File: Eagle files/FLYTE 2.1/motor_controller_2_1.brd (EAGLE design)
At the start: 80 x 53.6 mm, 38 parts, among them J1 XT60-M, U1 MIC29302WU-TRTO-263-5_MCH-M, U2 MIC29302WU-TRTO-263-5_MCH-M

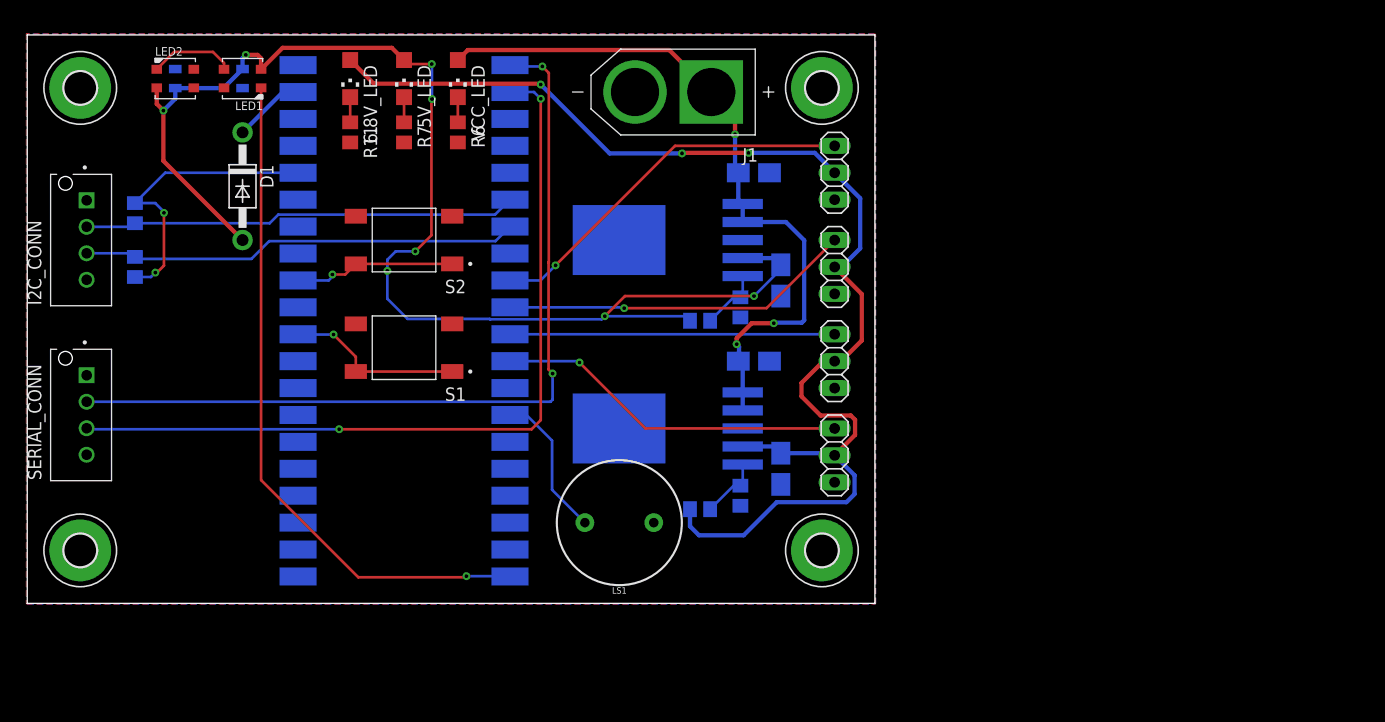
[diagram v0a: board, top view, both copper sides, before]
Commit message: motor controller v2.1
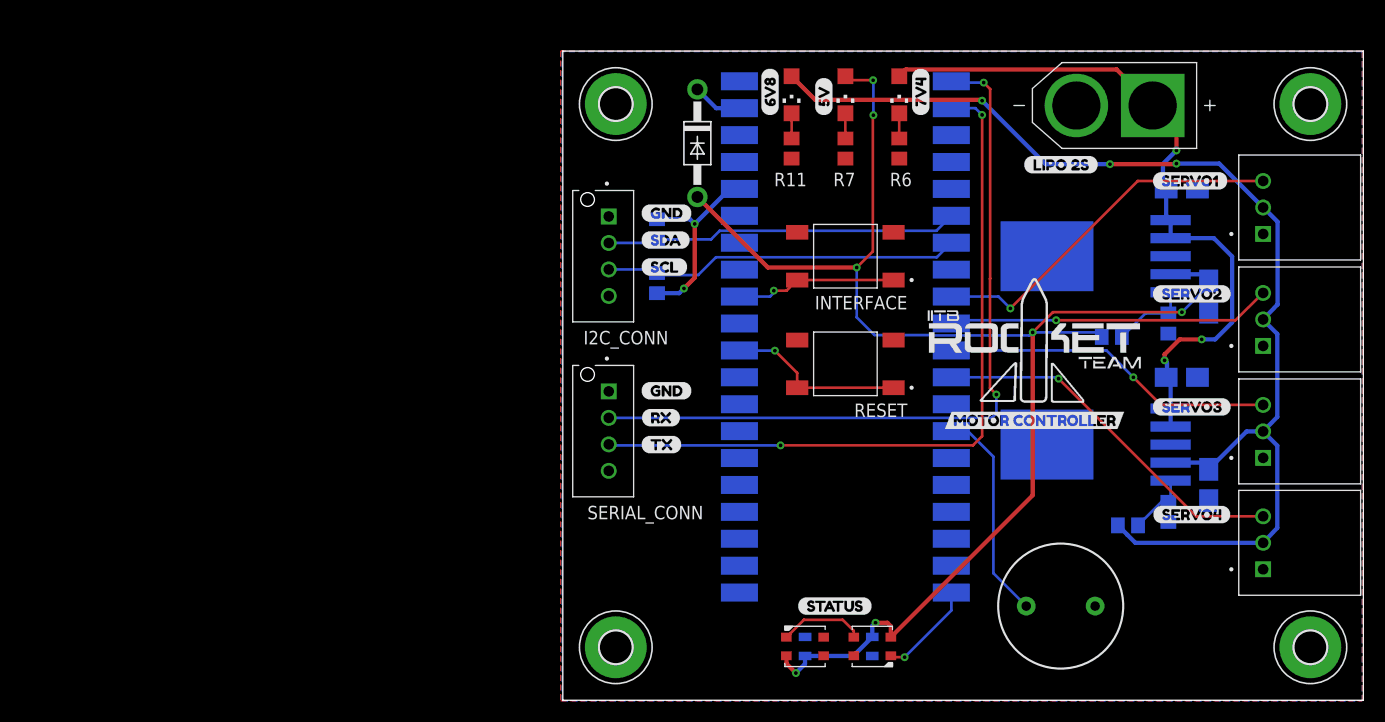
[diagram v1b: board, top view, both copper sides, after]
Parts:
- removed S1, S2: TS04-66-95-BK-100-SMT, TS04-66-95-BK-100-SMT:SW_TS04-66-95-BK-100-SMT
- removed SERVO1, SERVO2, SERVO3, SERVO4: (no value), pinhead:1X03
- added INTERFACE, RESET: TS04-66-95-BK-100-SMT, TS04-66-95-BK-100-SMT:SW_TS04-66-95-BK-100-SMT
- added J2, J3, J4, J5: S3B-XH-A(LF)(SN), S3B-XH-A_LF__SN_:JST_S3B-XH-A(LF)(SN)
- added U$1: (no value), servo1_label:SERVO10
- added U$10: (no value), tx_label:TX0
- added U$11: (no value), lipo_2s_label:LIPO_2S0
- added U$12: (no value), 5v_label:5V0
- added U$13: (no value), 7v4_label:7V40
- added U$14: (no value), 6v8_label:6V80
- added U$15: (no value), status_label:STATUS0
- added U$16: (no value), motor_controller_label:MOTOR_CONTROLLER0
- added U$2: (no value), servo2_label:SERVO20
- added U$3: (no value), servo3_label:SERVO30
- added U$4: (no value), servo4_label:SERVO40
- added U$5: (no value), sda_label:SDA0
- added U$6: (no value), scl_label:SCL0
- added U$7, U$8: (no value), gnd_label:GND0
- added U$9: (no value), rx_label:RX0
- moved C4 80.0 mm to (73.4, 2.29)
- moved LED2 80.0 mm to (73.4, 2.29)
- moved C3 80.0 mm to (79.8, 2.29)
- moved LED1 80.0 mm to (79.8, 2.29)
- moved H3 51.4 mm to (55.5, 2.21)
- moved H2 50.6 mm to (55.5, 53.5)
- moved I2C_CONN 49.3 mm to (54.4, 39.1)
- moved SERIAL_CONN 49.3 mm to (54.4, 22.6)
- moved R3 49.3 mm to (59.4, 36.6)
- moved R4 49.3 mm to (59.4, 41.7)
- moved H4 47.0 mm to (121.1, 2.21)
- moved H1 46.1 mm to (121.1, 53.5)
- moved D1 43.1 mm to (63.2, 49.8)
- moved LS1 42.4 mm to (97.5, 6.10)
- moved PICO 41.7 mm to (78.5, 30.2)
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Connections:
- net 6.8V: now also J2.2, J3.2, J4.2, J5.2; no longer SERVO1.2, SERVO2.2, SERVO3.2, SERVO4.2
- net GND: now also INTERFACE.2, INTERFACE.4, J2.1, J3.1, J4.1, J5.1, RESET.2, RESET.4; no longer S1.2, S1.4, S2.2, S2.4, SERVO1.1, SERVO2.1, SERVO3.1, SERVO4.1
- net N$2: now also RESET.1, RESET.3; no longer S1.1, S1.3
- net N$3: now also INTERFACE.1, INTERFACE.3; no longer S2.1, S2.3
- net SERVO1: now also J2.3; no longer SERVO1.3
- net SERVO2: now also J3.3; no longer SERVO2.3
- net SERVO3: now also J4.3; no longer SERVO3.3
- net SERVO4: now also J5.3; no longer SERVO4.3
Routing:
- net LED: track 65.7 -> 9.28 mm
- net 5V: track 126.4 -> 139.9 mm, vias 8 -> 7
- net 6.8V: track 120.8 -> 109.6 mm
- net 3V3: track 28.0 -> 18.6 mm
- net SDA0: track 41.0 -> 33.4 mm
- net SCL0: track 41.4 -> 33.8 mm
- net SER_RX: track 76.7 -> 69.1 mm
- net SER_TX: track 79.0 -> 71.6 mm
- net BUZZER: track 14.0 -> 20.4 mm
- net SERVO2: track 33.3 -> 30.6 mm
- net N$1: track 6.82 -> 4.71 mm
- net SERVO4: track 33.3 -> 34.9 mm
- net N$14: track 5.92 -> 7.44 mm
- net SERVO1: track 35.9 -> 34.9 mm
- net SERVO3: track 30.6 -> 31.6 mm, vias 0 -> 1
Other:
- board size 80 x 53.6 mm -> 75.6 x 61.3 mm
- board text added: "R10"

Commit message: flyte done
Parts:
- 5V_LED, 6.8V_LED, VCC_LED: device adafruit:CHIPLED_1206 -> led:CHIPLED_1206

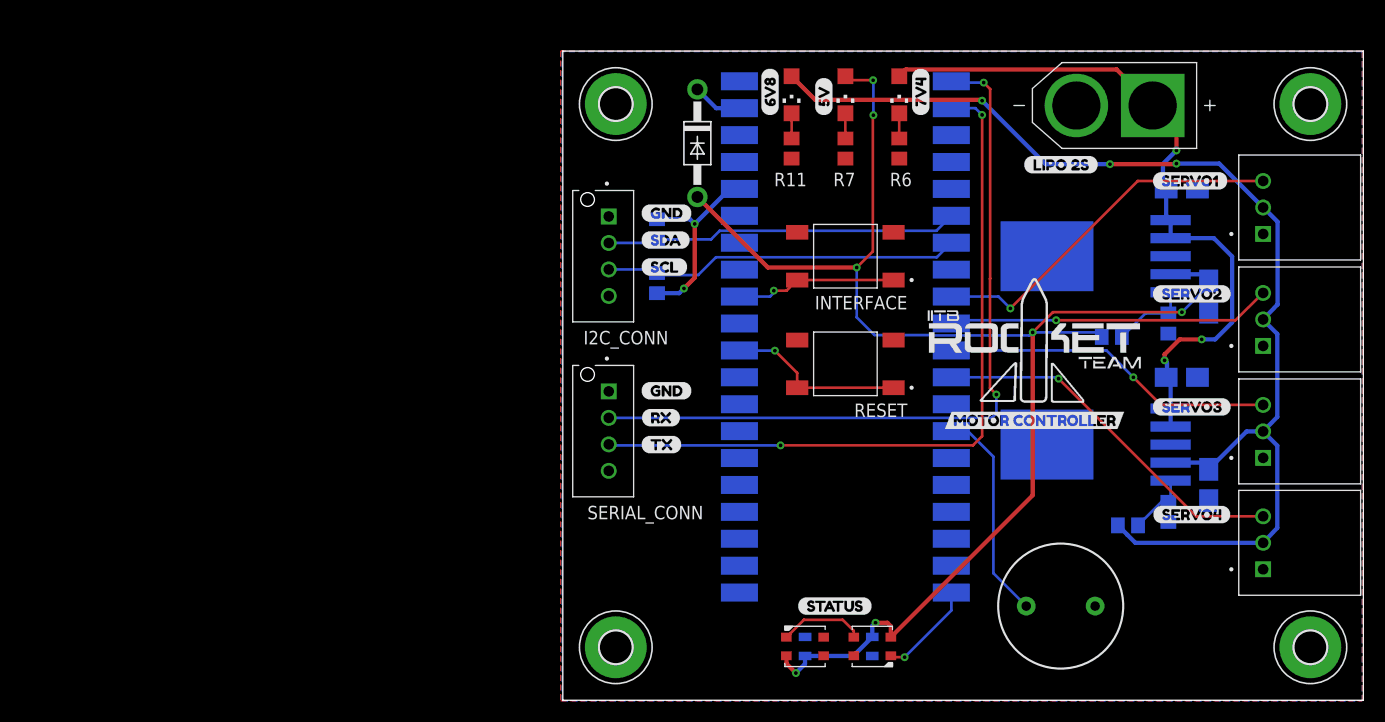
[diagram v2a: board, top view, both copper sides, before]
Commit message: .
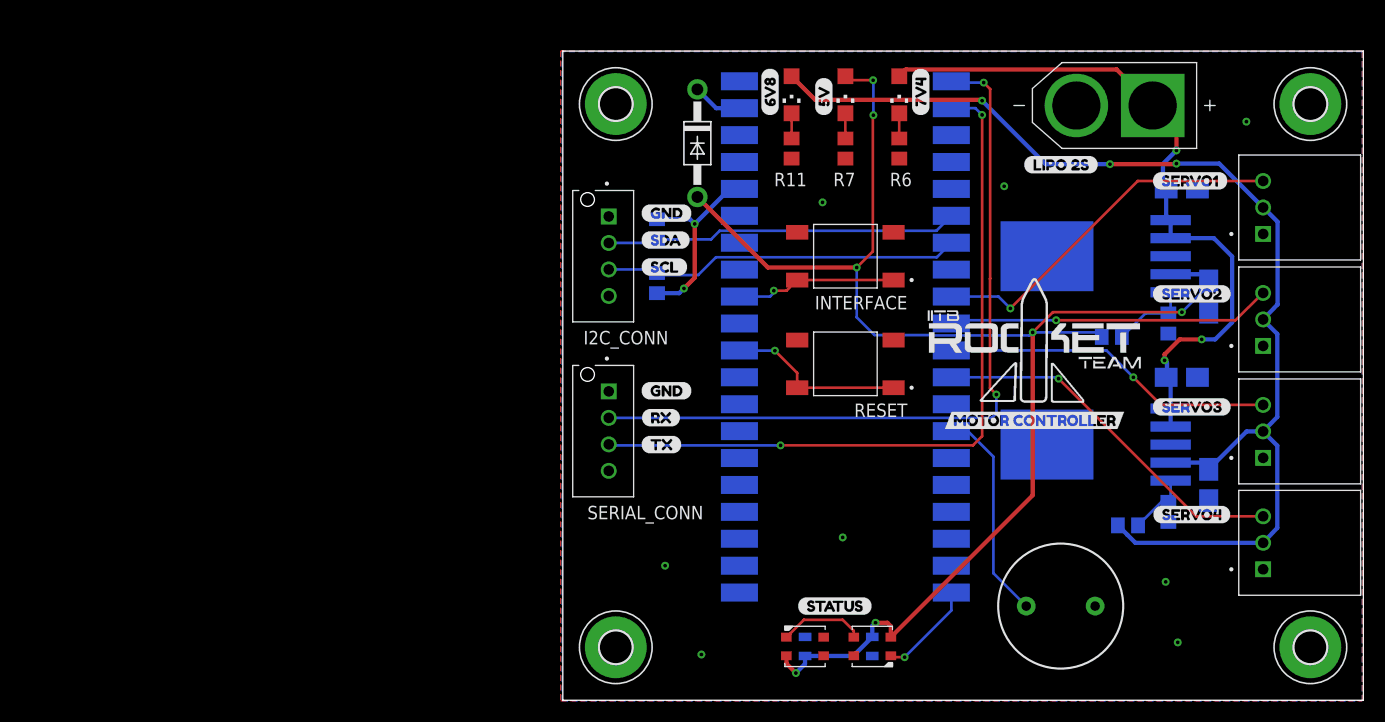
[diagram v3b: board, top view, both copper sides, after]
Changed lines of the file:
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@@
 </layers>
 <board>
-<fusionsync huburn="a.YnVzaW5lc3M6aWl0YjUzNQ" projecturn="a.YnVzaW5lc3M6aWl0YjUzNSNEMjAyMjA3MjU1NDIwMjEzNzY" f3durn="urn:adsk.wipprod:dm.lineage:8IMc14VtSl-5fDwUJquSpw" pcbguid="" lastpulledtime="" lastsyncedchangeguid="" latestrevisionid="a0f8438c-b738-4322-bdc5-6236827b66e7" lastsyncedrevisionid="a0f8438c-b738-4322-bdc5-6236827b66e7" lastboardhashguid="21d1f3f7-0f8b-bc3e-4432-33a0da882c0f" lastpushedtime="2024-05-08T04:04:01Z" linktopcb3d="true"/>
+<fusionsync huburn="a.YnVzaW5lc3M6aWl0YjUzNQ" projecturn="a.YnVzaW5lc3M6aWl0YjUzNSNEMjAyMjA3MjU1NDIwMjEzNzY" f3durn="urn:adsk.wipprod:dm.lineage:8IMc14VtSl-5fDwUJquSpw" pcbguid="" lastpulledtime="" lastsyncedchangeguid="" latestrevisionid="a0f8438c-b738-4322-bdc5-6236827b66e7" lastsyncedrevisionid="a0f8438c-b738-4322-bdc5-6236827b66e7" lastboardhashguid="21d1f3f7-0f8b-bc3e-4432-33a0da882c0f" lastpushedtime="2024-05-08T04:04:01Z" linktopcb3d="false"/>
 <plain>
 <wire x1="50.546" y1="-2.794" x2="126.101" y2="-2.794" width="0" layer="20"/>
@@
 <wire x1="72.136" y1="52.606" x2="72.136" y2="50.226" width="0.254" layer="1"/>
 </signal>
+<signal name="N$4">
+<via x="60.198" y="9.906" extent="1-16" drill="0.35"/>
+</signal>
+<signal name="N$6">
+<via x="76.962" y="12.573" extent="1-16" drill="0.35"/>
+</signal>
+<signal name="N$11">
+<via x="108.585" y="2.667" extent="1-16" drill="0.35"/>
+</signal>
+<signal name="N$12">
+<via x="107.442" y="8.382" extent="1-16" drill="0.35"/>
+</signal>
+<signal name="N$13">
+<via x="92.202" y="45.72" extent="1-16" drill="0.35"/>
+</signal>
+<signal name="N$15">
+<via x="115.062" y="51.816" extent="1-16" drill="0.35"/>
+</signal>
+<signal name="N$16">
+<via x="75.057" y="44.196" extent="1-16" drill="0.35"/>
+</signal>
+<signal name="N$17">
+<via x="63.627" y="1.524" extent="1-16" drill="0.35"/>
+</signal>
 </signals>

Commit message: .
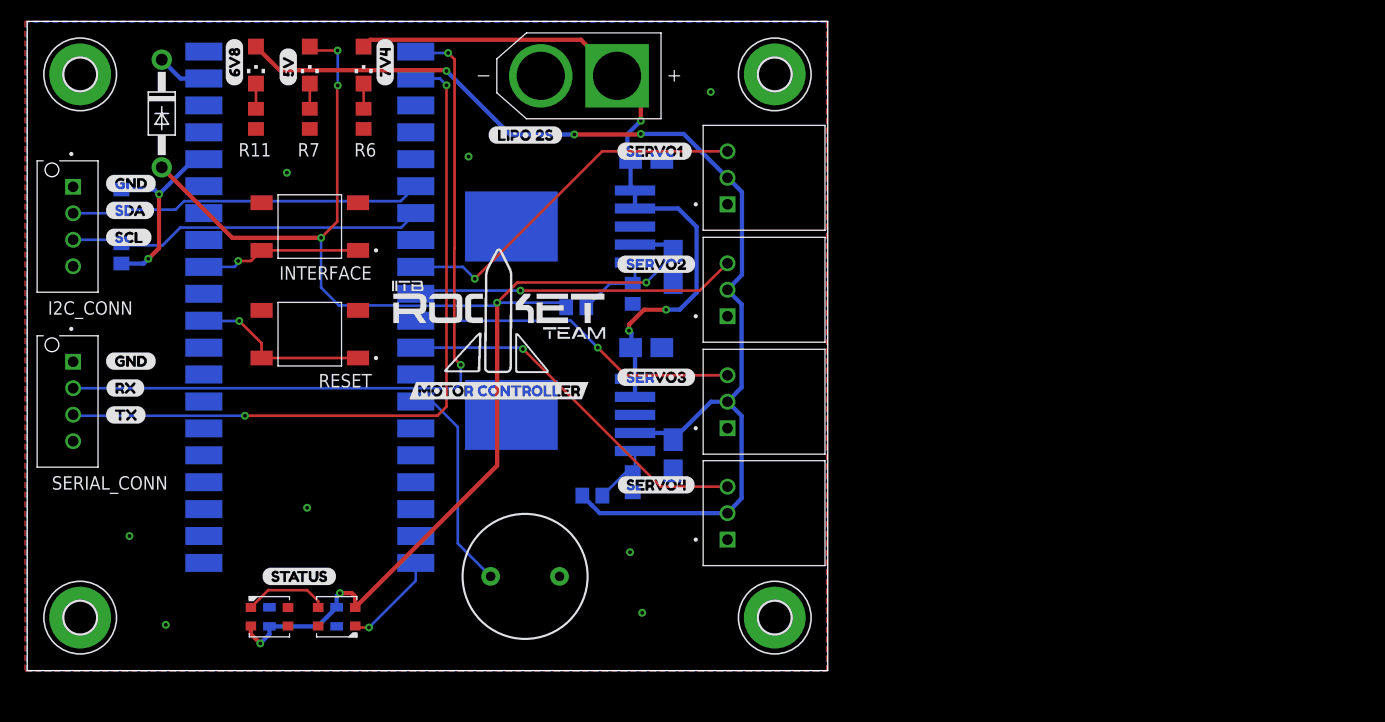
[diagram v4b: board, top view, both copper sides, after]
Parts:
- moved R6 50.6 mm to (31.7, 52.1)
- moved VCC_LED 50.6 mm to (31.7, 57.2)
- moved C4 50.6 mm to (22.9, 5.09)
- moved D1 50.6 mm to (12.7, 52.6)
- moved I2C_CONN 50.6 mm to (3.81, 41.9)
- moved LED2 50.6 mm to (22.9, 5.09)
- moved LS1 50.6 mm to (47.0, 8.90)
- moved PICO 50.6 mm to (27.9, 33.0)
- moved SERIAL_CONN 50.6 mm to (3.81, 25.4)
- moved U$11 50.6 mm to (43.4, 50.6)
- moved U$13 50.6 mm to (33.8, 55.1)
- moved U$15 50.6 mm to (22.1, 8.90)
- moved 5V_LED 50.6 mm to (26.7, 57.2)
- moved 6.8V_LED 50.6 mm to (21.6, 57.2)
- moved C1 50.6 mm to (58.4, 48.3)
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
